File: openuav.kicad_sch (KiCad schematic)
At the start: 70 parts, among them J1 Conn_01x01, J10 Conn_01x01, J11 Conn_01x01, J12 Conn_01x01, J13 Conn_01x01, J14 Conn_01x01, J15 Conn_01x01, J16 Conn_01x01, J17 Conn_01x01, J18 Conn_01x01, J19 Conn_01x01, J2 Conn_01x01, J20 Conn_01x01, J21 Conn_01x01, J22 Conn_01x01, J23 Conn_01x01, J24 Conn_01x01, J25 Conn_01x01, J26 Conn_01x01, J27 Conn_01x01, J28 Conn_01x01, J29 Conn_01x01, J3 Conn_01x01, J30 Conn_01x01, J31 Conn_01x01, J4 Conn_01x01, J5 Conn_01x01, J6 Conn_01x01, J7 Conn_01x01, J8 Conn_01x01, J9 Conn_01x01, J99 USB_C_Receptacle_USB2.0, SW1 SW_Push, U1 STM32G474CETx, U2 BMI270, U3 BMP280, U5 TPS54202DDC, U6 W25N01GVZEIG, U7 XC6206P332MR

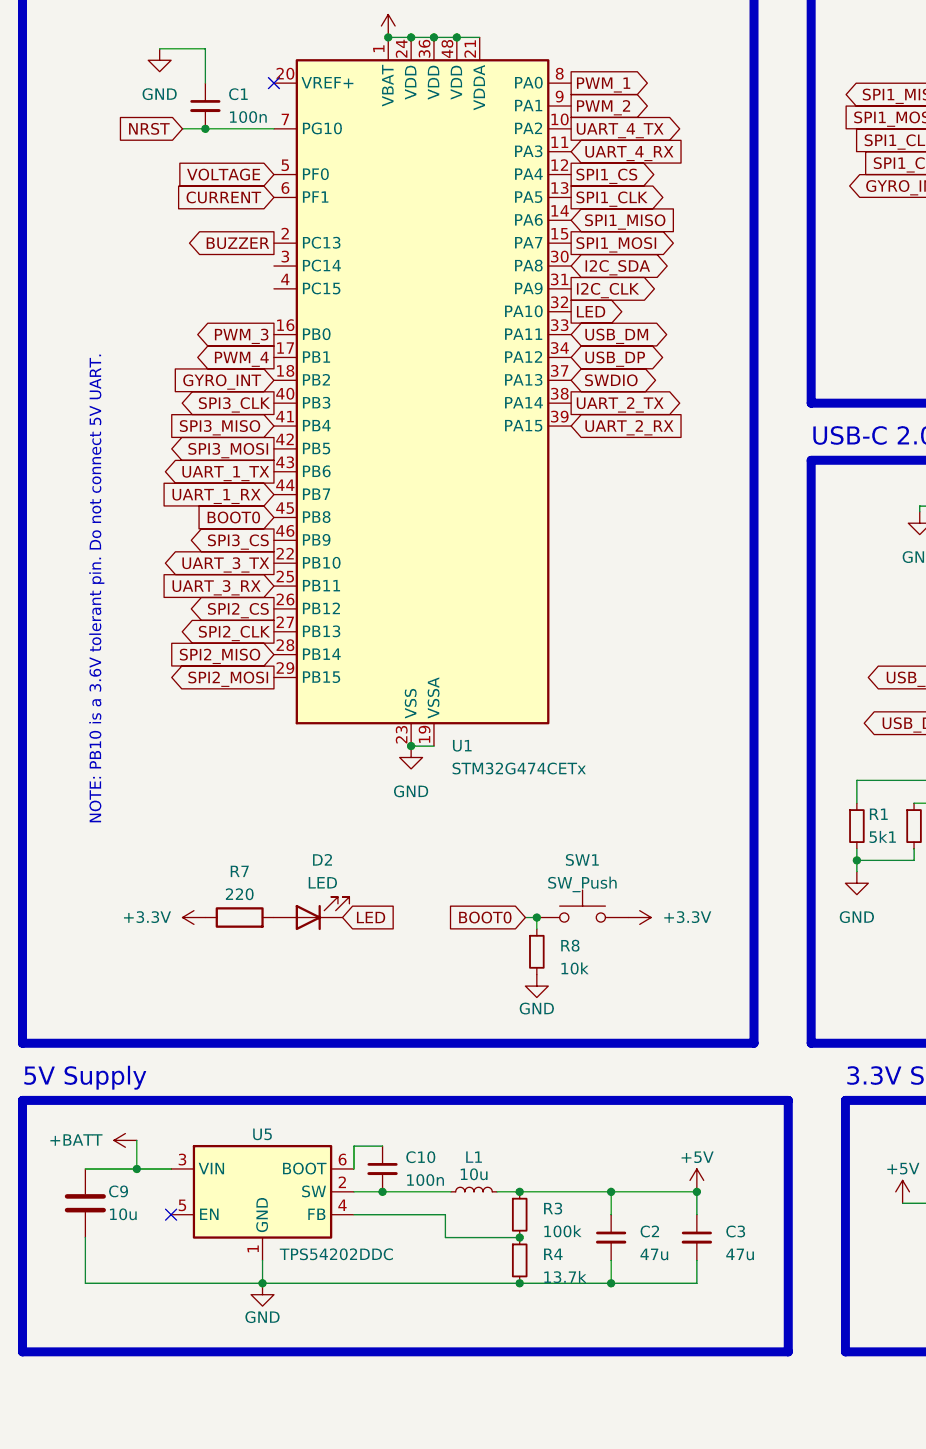
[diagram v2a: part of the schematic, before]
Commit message: routing
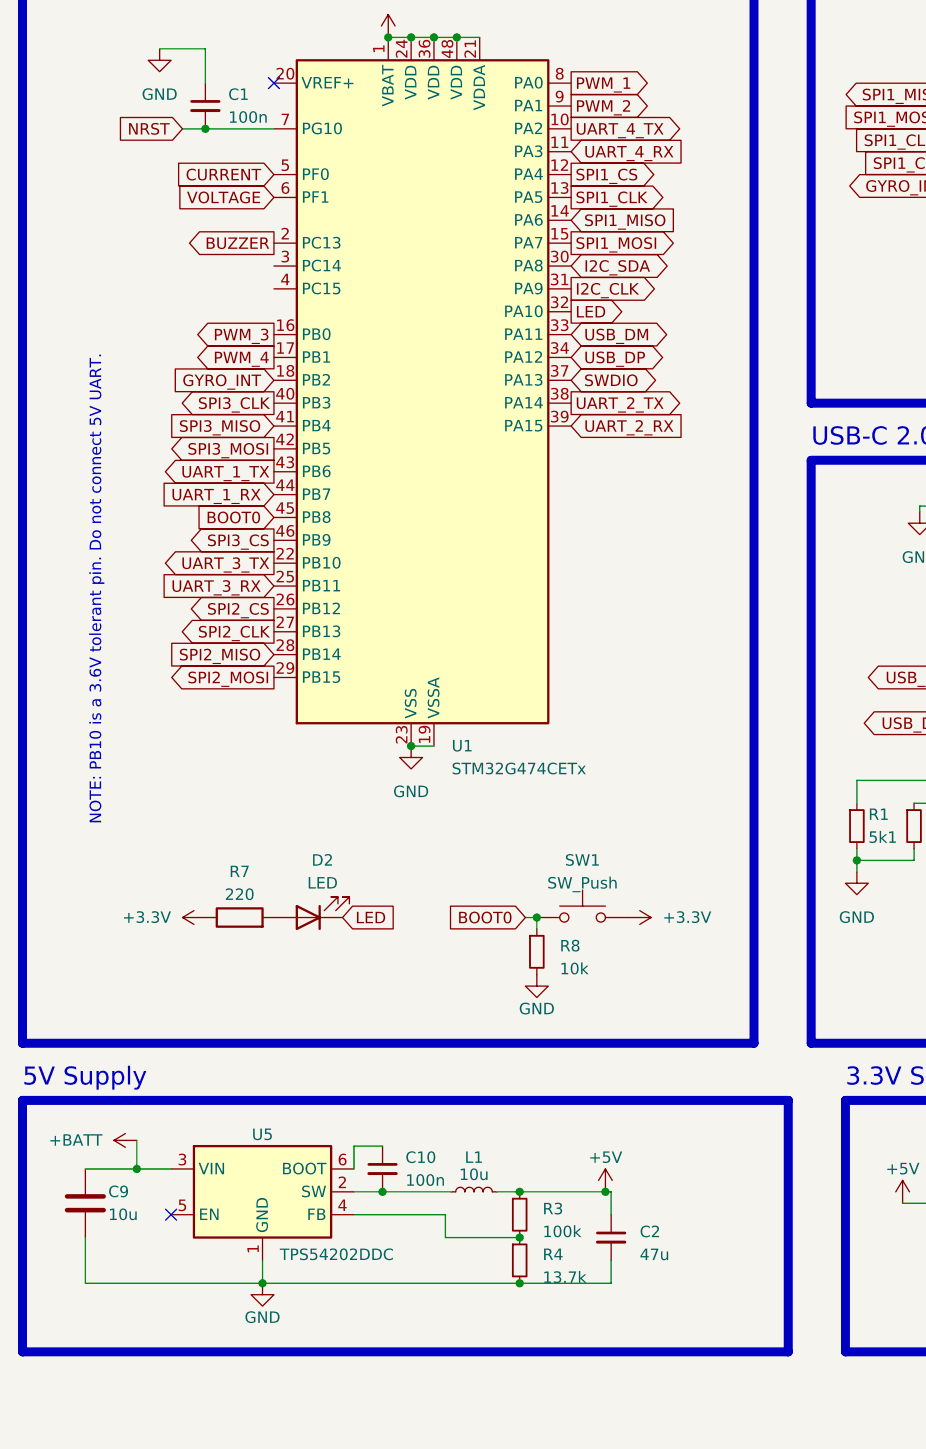
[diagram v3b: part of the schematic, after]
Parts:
- removed C3: 47u, Capacitor_SMD:C_1206_3216Metric, symbol Device:C_Small
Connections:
- net CURRENT: now also U1.5 (PF0); no longer U1.6 (PF1)
- net VOLTAGE: now also U1.6 (PF1); no longer U1.5 (PF0)
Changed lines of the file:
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@@
   (junction (at 121.92 115.57) (diameter 0) (color 0 0 0 0)
   )
-  (junction (at 81.915 177.8) (diameter 0) (color 0 0 0 0)
-  )
   (junction (at 138.43 168.91) (diameter 0) (color 0 0 0 0)
   )
@@
   (junction (at 224.79 173.99) (diameter 0) (color 0 0 0 0)
   )
+  (junction (at 81.28 167.64) (diameter 0) (color 0 0 0 0)
+  )
   (junction (at 71.755 172.72) (diameter 0) (color 0 0 0 0)
   )
@@
   (junction (at 184.15 168.91) (diameter 0) (color 0 0 0 0)
   )
-  (junction (at 81.915 167.64) (diameter 0) (color 0 0 0 0)
-  )
   (junction (at 194.31 168.91) (diameter 0) (color 0 0 0 0)
   )
@@
   )
   (junction (at 57.15 39.37) (diameter 0) (color 0 0 0 0)
-  )
-  (junction (at 91.44 167.64) (diameter 0) (color 0 0 0 0)
   )
   (junction (at 59.69 118.11) (diameter 0) (color 0 0 0 0)
@@
     (stroke (width 0) (type default))
   )
+  (wire (pts (xy 81.28 167.64) (xy 81.915 167.64))
+    (stroke (width 0) (type default))
+  )
   (wire (pts (xy 109.22 121.92) (xy 109.22 124.46))
     (stroke (width 0) (type default))
@@
     (stroke (width 0) (type default))
   )
-  (wire (pts (xy 81.915 167.64) (xy 91.44 167.64))
-    (stroke (width 0) (type default))
-  )
   (wire (pts (xy 64.77 39.37) (xy 67.31 39.37))
     (stroke (width 0) (type default))
@@
     (stroke (width 0) (type default))
   )
-  (wire (pts (xy 71.755 167.64) (xy 81.915 167.64))
-    (stroke (width 0) (type default))
-  )
-  (wire (pts (xy 91.44 175.26) (xy 91.44 177.8))
+  (wire (pts (xy 71.755 167.64) (xy 81.28 167.64))
     (stroke (width 0) (type default))
   )
@@
     (stroke (width 0) (type default))
   )
-  (wire (pts (xy 91.44 167.64) (xy 91.44 170.18))
-    (stroke (width 0) (type default))
-  )
   (wire (pts (xy 184.15 173.99) (xy 194.31 173.99))
     (stroke (width 0) (type default))
@@
   )
   (wire (pts (xy 224.79 168.91) (xy 234.95 168.91))
-    (stroke (width 0) (type default))
-  )
-  (wire (pts (xy 81.915 177.8) (xy 91.44 177.8))
     (stroke (width 0) (type default))
   )
@@
     )
   )
-  (global_label "CURRENT" (shape input) (at 44.45 57.15 180) (fields_autoplaced)
-    (effects (font (size 1.27 1.27)) (justify right))
-    (property "Intersheetrefs" "${INTERSHEET_REFS}" (at 32.9566 57.15 0)
+  (global_label "CURRENT" (shape input) (at 44.45 54.61 180) (fields_autoplaced)
+    (effects (font (size 1.27 1.27)) (justify right))
+    (property "Intersheetrefs" "${INTERSHEET_REFS}" (at 32.9566 54.61 0)
       (effects (font (size 1.27 1.27)) (justify right) hide)
     )
@@
     )
   )
-  (global_label "VOLTAGE" (shape input) (at 44.45 54.61 180) (fields_autoplaced)
-    (effects (font (size 1.27 1.27)) (justify right))
-    (property "Intersheetrefs" "${INTERSHEET_REFS}" (at 33.6218 54.61 0)
+  (global_label "VOLTAGE" (shape input) (at 44.45 57.15 180) (fields_autoplaced)
+    (effects (font (size 1.27 1.27)) (justify right))
+    (property "Intersheetrefs" "${INTERSHEET_REFS}" (at 33.6218 57.15 0)
       (effects (font (size 1.27 1.27)) (justify right) hide)
     )
@@
     )
   )
-  (symbol (lib_id "power:+5V") (at 91.44 167.64 0) (unit 1)
+  (symbol (lib_id "power:+5V") (at 81.28 167.64 0) (unit 1)
     (in_bom yes) (on_board yes) (dnp no) (fields_autoplaced)
-    (property "Reference" "#PWR07" (at 91.44 171.45 0)
-      (effects (font (size 1.27 1.27)) hide)
-    )
-    (property "Value" "+5V" (at 91.44 163.83 0)
+    (property "Reference" "#PWR07" (at 81.28 171.45 0)
+      (effects (font (size 1.27 1.27)) hide)
+    )
+    (property "Value" "+5V" (at 81.28 163.83 0)
       (effects (font (size 1.27 1.27)))
     )
-    (property "Footprint" "" (at 91.44 167.64 0)
-      (effects (font (size 1.27 1.27)) hide)
-    )
-    (property "Datasheet" "" (at 91.44 167.64 0)
+    (property "Footprint" "" (at 81.28 167.64 0)
+      (effects (font (size 1.27 1.27)) hide)
+    )
+    (property "Datasheet" "" (at 81.28 167.64 0)
       (effects (font (size 1.27 1.27)) hide)
     )
@@
         )
       )
-    )
-  )
-  (symbol (lib_id "Device:C_Small") (at 91.44 172.72 0) (unit 1)
-    (in_bom yes) (on_board yes) (dnp no) (fields_autoplaced)
-    (property "Reference" "C3" (at 94.615 172.0913 0)
-      (effects (font (size 1.27 1.27)) (justify left))
-    )
-    (property "Value" "47u" (at 94.615 174.6313 0)
-      (effects (font (size 1.27 1.27)) (justify left))
-    )
-    (property "Footprint" "Capacitor_SMD:C_1206_3216Metric" (at 91.44 172.72 0)
-      (effects (font (size 1.27 1.27)) hide)
-    )
-    (property "Datasheet" "~" (at 91.44 172.72 0)
-      (effects (font (size 1.27 1.27)) hide)
-    )
-    (property "LCSC" "C96123" (at 91.44 172.72 0)
-      (effects (font (size 1.27 1.27)) hide)
-    )
-    (pin "1")
-    (pin "2")
-    (instances
-      (project "openuav"
-        (path "/e63e39d7-6ac0-4ffd-8aa3-1841a4541b55"
-          (reference "C3") (unit 1)
-        )
-      )
